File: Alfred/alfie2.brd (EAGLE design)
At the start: 50 x 50 mm, 16 parts, among them IC1 7805TV, X3 04-JST-B4B-XH-A

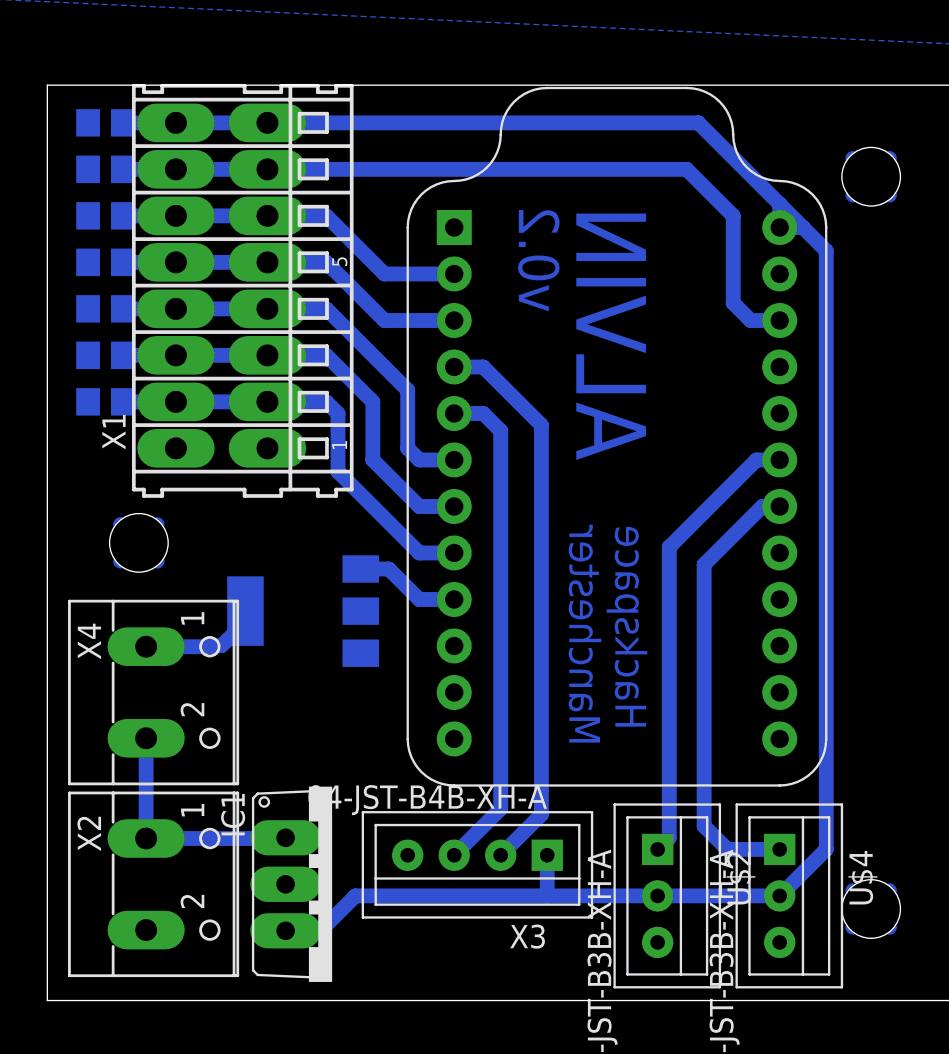
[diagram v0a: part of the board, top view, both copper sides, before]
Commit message: alfie2 v0.2 - visicut laser cutter file
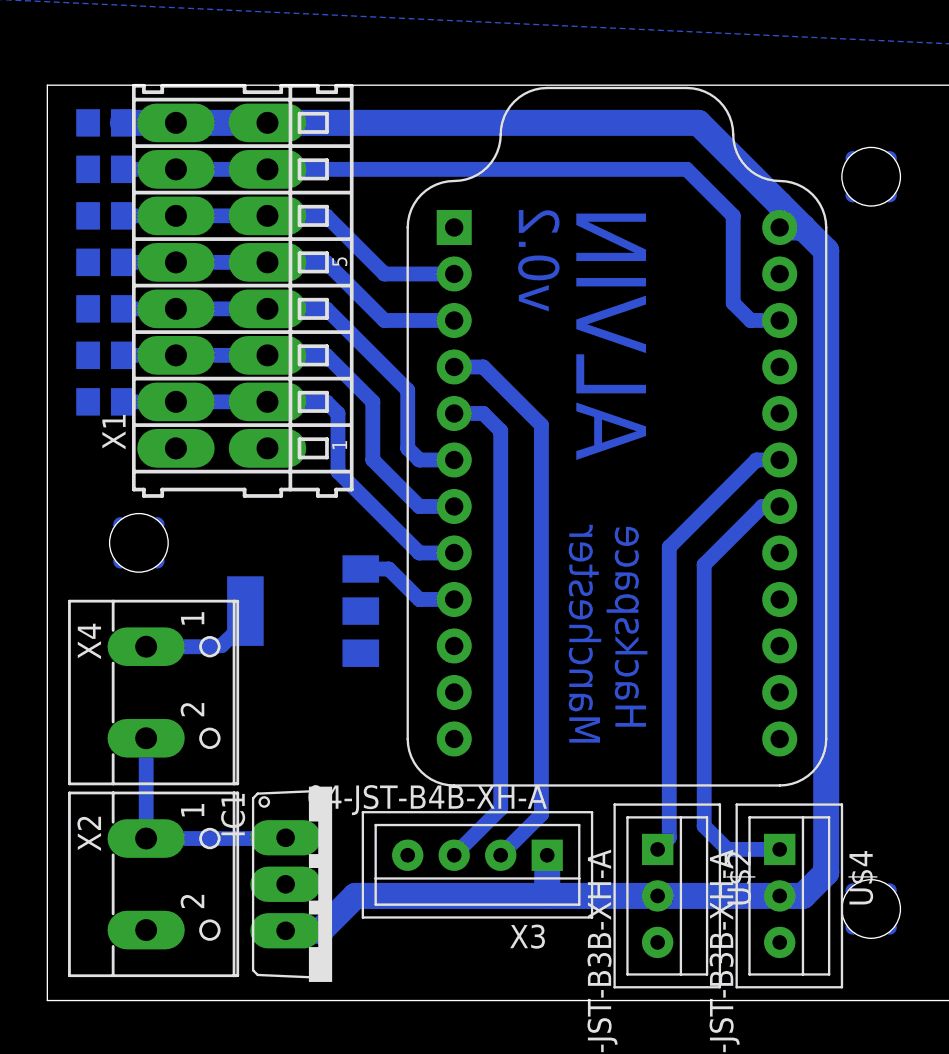
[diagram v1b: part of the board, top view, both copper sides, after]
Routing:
- net +5V: track 110.1 -> 110.9 mm
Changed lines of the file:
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@@
 <setting verticaltext="up"/>
 </settings>
-<grid distance="1" unitdist="mm" unit="mm" style="lines" multiple="1" display="yes" altdistance="0.025" altunitdist="inch" altunit="inch"/>
+<grid distance="12.5" unitdist="mil" unit="mil" style="lines" multiple="1" display="yes" altdistance="0.025" altunitdist="inch" altunit="inch"/>
 <layers>
 <layer number="1" name="Top" color="4" fill="1" visible="yes" active="yes"/>
@@
 <contactref element="X1" pad="B8"/>
 <contactref element="C9" pad="1"/>
-<wire x1="12.025" y1="47.9425" x2="4.125" y2="47.9425" width="0.8128" layer="16"/>
-<wire x1="42.545" y1="8.255" x2="42.545" y2="40.9575" width="0.8128" layer="16"/>
-<wire x1="35.56" y1="47.9425" x2="12.025" y2="47.9425" width="0.8128" layer="16"/>
+<wire x1="12.025" y1="47.9425" x2="4.125" y2="47.9425" width="1.4224" layer="16"/>
+<wire x1="42.545" y1="6.985" x2="42.545" y2="40.9575" width="1.4224" layer="16"/>
+<wire x1="35.56" y1="47.9425" x2="12.025" y2="47.9425" width="1.4224" layer="16"/>
 <wire x1="40.005" y1="42.2275" x2="40.0075" y2="42.2275" width="0.8128" layer="16"/>
-<wire x1="42.545" y1="40.9575" x2="41.275" y2="42.2275" width="0.8128" layer="16"/>
-<wire x1="40.005" y1="43.4975" x2="35.56" y2="47.9425" width="0.8128" layer="16"/>
-<wire x1="40.005" y1="42.2275" x2="41.275" y2="42.2275" width="0.8128" layer="16"/>
-<wire x1="41.275" y1="42.2275" x2="40.005" y2="43.4975" width="0.8128" layer="16"/>
+<wire x1="42.545" y1="40.9575" x2="41.275" y2="42.2275" width="1.4224" layer="16"/>
+<wire x1="40.005" y1="43.4975" x2="35.56" y2="47.9425" width="1.4224" layer="16"/>
+<wire x1="40.005" y1="42.2275" x2="41.275" y2="42.2275" width="1.4224" layer="16"/>
+<wire x1="41.275" y1="42.2275" x2="40.005" y2="43.4975" width="1.4224" layer="16"/>
 <wire x1="40.005" y1="43.4975" x2="40.005" y2="42.2275" width="0.8128" layer="16"/>
 <contactref element="X3" pad="P$1"/>
 <contactref element="U$2" pad="P$2"/>
 <contactref element="IC1" pad="3"/>
-<wire x1="16.8275" y1="5.715" x2="27.305" y2="5.715" width="0.8128" layer="16"/>
-<wire x1="27.305" y1="5.715" x2="33.3375" y2="5.715" width="0.8128" layer="16"/>
+<wire x1="16.8275" y1="5.715" x2="27.305" y2="5.715" width="1.4224" layer="16"/>
+<wire x1="27.305" y1="5.715" x2="33.3375" y2="5.715" width="1.4224" layer="16"/>
 <contactref element="U$4" pad="P$2"/>
-<wire x1="27.305" y1="7.9375" x2="27.305" y2="5.715" width="0.8128" layer="16"/>
-<wire x1="13.0175" y1="3.81" x2="14.9225" y2="3.81" width="0.8128" layer="16"/>
-<wire x1="14.9225" y1="3.81" x2="16.8275" y2="5.715" width="0.8128" layer="16"/>
-<wire x1="33.3375" y1="5.715" x2="40.005" y2="5.715" width="0.8128" layer="16"/>
-<wire x1="40.005" y1="5.715" x2="42.545" y2="8.255" width="0.8128" layer="16"/>
+<wire x1="27.305" y1="7.9375" x2="27.305" y2="5.715" width="1.4224" layer="16"/>
+<wire x1="13.0175" y1="3.81" x2="14.9225" y2="3.81" width="1.4224" layer="16"/>
+<wire x1="14.9225" y1="3.81" x2="16.8275" y2="5.715" width="1.4224" layer="16"/>
+<wire x1="33.3375" y1="5.715" x2="40.005" y2="5.715" width="1.4224" layer="16"/>
+<wire x1="40.005" y1="5.715" x2="41.275" y2="5.715" width="1.4224" layer="16"/>
+<wire x1="41.275" y1="5.715" x2="42.545" y2="6.985" width="1.4224" layer="16"/>
 </signal>
 <signal name="GND">
@@
 </signal>
 </signals>
+<errors>
+</errors>
 </board>
 </drawing>
